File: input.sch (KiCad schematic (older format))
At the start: 34 parts

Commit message: Add some part numbers, more changes
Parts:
- removed C?: 1nF, Capacitor_SMD:C_0603_1608Metric, symbol Device:C_Small
- removed D? (x2): 12V, Diode_SMD:D_SOD-523, symbol Device:D_Zener_Small
- removed J?: Jack-DC, Connector_BarrelJack:BarrelJack_Horizontal, symbol Connector:Jack-DC
- removed Q? (x3): 40V, Package_SO:Vishay_PowerPAK_1212-8_Single, symbol Device:Q_NMOS_SGD
- removed R?: 1M, Resistor_SMD:R_0603_1608Metric, symbol Device:R_Small
- removed R?: 100k, Resistor_SMD:R_0603_1608Metric, symbol Device:R_Small
- removed TP?: VBUS_DC, TestPoint:TestPoint_THTPad_D2.0mm_Drill1.0mm, symbol Connector:TestPoint_Small
- removed TP?: ACDRV2, TestPoint:TestPoint_THTPad_D2.0mm_Drill1.0mm, symbol Connector:TestPoint_Small
- C202, C203, C207: renamed from C?; JLC (none) -> 0603; LCSC (none) -> C14663; MPN (none) -> CC0603KRX7R9BB104
- R201, R202, R204, R205, R206: renamed from R?; JLC (none) -> 0603; LCSC (none) -> C25804
- U202: renamed from U?; JLC (none) -> MSOP-10_3.0x3.0x0.5P; LCSC (none) -> C11355; MPN (none) -> FSUSB42MUX
- gave numbers to parts that had none: 14
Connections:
- net labels removed: ACDRV2, VAC2
- wire segments 157 -> 124
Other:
- note removed: "XT60 or spring-loaded\nsockets here?"
- moved on the sheet: C201, C202, C203, C204, C205, C206, C207, D201, D202, J201, Q201, Q202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

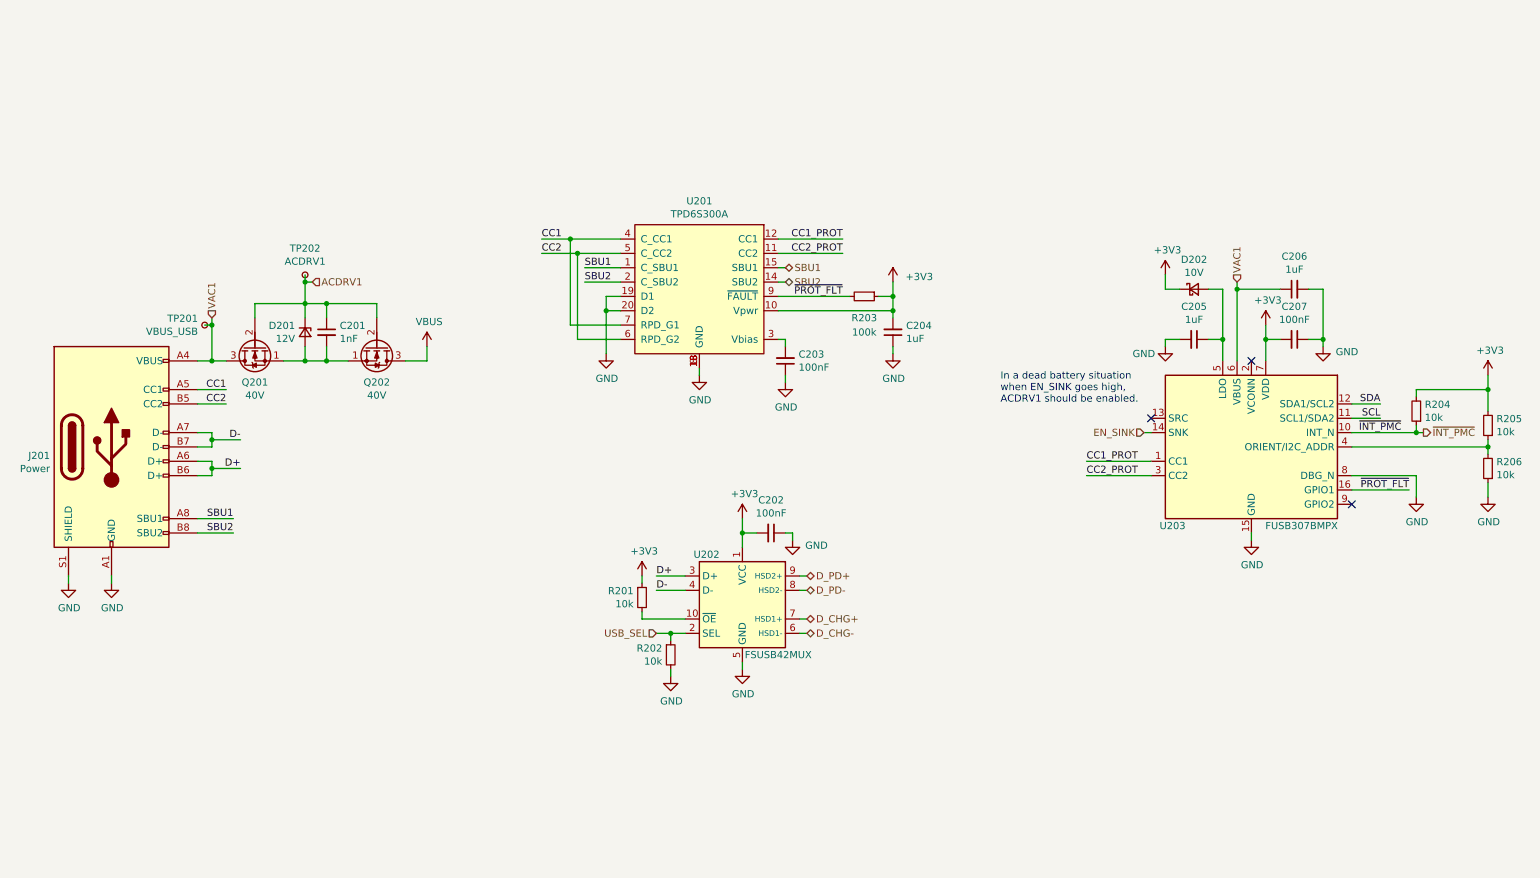
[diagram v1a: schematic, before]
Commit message: Schematic is done now
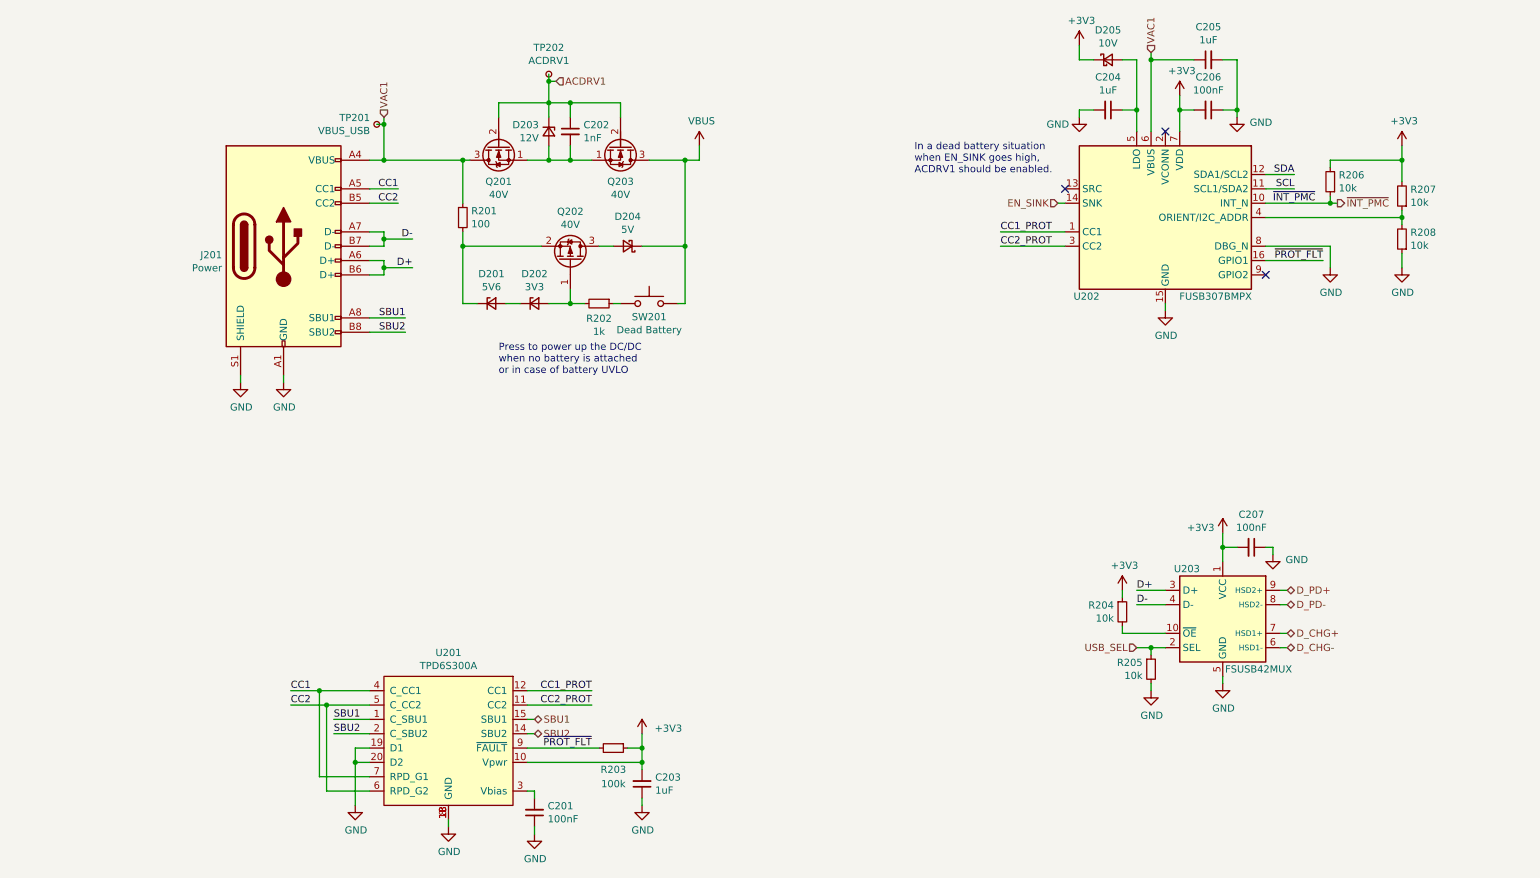
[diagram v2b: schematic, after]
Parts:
- added D201: 5V6, Diode_SMD:D_MiniMELF, symbol Device:D_Zener_Small
- added D202: 3V3, Diode_SMD:D_MiniMELF, symbol Device:D_Zener_Small
- added D204: 5V, Diode_SMD:D_SOD-123, symbol Device:D_Schottky_Small
- added Q202: 40V, Package_TO_SOT_SMD:SOT-23, symbol Device:Q_PMOS_GSD
- added R201: 100, Resistor_SMD:R_1206_3216Metric, symbol Device:R_Small
- added R202: 1k, Resistor_SMD:R_0603_1608Metric, symbol Device:R_Small
- added SW201: Dead Battery, Automated:SW_SPST_PTS636_G, symbol Switch:SW_Push
- C202: renamed from C201; footprint Capacitor_SMD:C_0603_1608Metric -> Capacitor_SMD:C_0402_1005Metric; JLC (none) -> 0402; LCSC (none) -> C1523
- renumbered C203 to C201, C204 to C203, C205 to C204, C206 to C205, C207 to C206, C202 to C207, D201 to D203, D202 to D205, Q202 to Q203, R201 to R204, R202 to R205, R204 to R206, R205 to R207, R206 to R208, U203 to U202, U202 to U203
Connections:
- net VAC1: now also R201.1
- net VBUS: now also D204.1 (K), SW201.2
- new net: D204.2 (A), Q202.3 (D)
- new net: D202.2 (A), Q202.1 (G), R202.2
- new net: D201.1 (K), Q202.2 (S), R201.2
- new net: R202.1, SW201.1
- new net: D201.2 (A), D202.1 (K)
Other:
- note added: "Press to power up the DC/DC \nwhen no battery is attached\nor in case of battery UVLO"
- moved on the sheet: C201, C202, C203, C204, C205, C206, C207, D203, D205, J201, Q201, Q203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

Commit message: Start with layout
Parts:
- C207: footprint Capacitor_SMD:C_0603_1608Metric -> Capacitor_SMD:C_0402_1005Metric; JLC 0603 -> 0402; LCSC C14663 -> (none); MPN CC0603KRX7R9BB104 -> (none)
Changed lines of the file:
@@
 F 0 "C207" V 8921 4650 50  0000 C CNN
 F 1 "100nF" V 9012 4650 50  0000 C CNN
-F 2 "Capacitor_SMD:C_0603_1608Metric" H 9150 4650 50  0001 C CNN
+F 2 "Capacitor_SMD:C_0402_1005Metric" H 9150 4650 50  0001 C CNN
 F 3 "~" H 9150 4650 50  0001 C CNN
-F 4 "0603" H 9150 4650 50  0001 C CNN "JLC"
-F 5 "C14663" H 9150 4650 50  0001 C CNN "LCSC"
-F 6 "CC0603KRX7R9BB104" H 9150 4650 50  0001 C CNN "MPN"
+F 4 "0402" H 9150 4650 50  0001 C CNN "JLC"
+F 5 "" H 9150 4650 50  0001 C CNN "LCSC"
+F 6 "" H 9150 4650 50  0001 C CNN "MPN"
 	1    9150 4650
 	0    1    1    0
